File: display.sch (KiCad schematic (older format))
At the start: 122 parts, among them P1 CONN_02X14, P2 CONN_02X15, Q1 BC846, Q10 BC846, Q11 BC856, Q12 BC856, Q13 BC846, Q14 BC846, Q15 BC856, Q16 BC856, Q17 BC846, Q18 BC846, Q19 BC856, Q2 BC846, Q20 BC856, Q21 BC846, Q22 BC846, Q23 BC856, Q24 BC856, Q25 BC846, Q26 BC846, Q27 BC856, Q28 BC856, Q29 BC846, Q3 BC856, Q30 BC846, Q31 BC856, Q32 BC856, Q33 BC846, Q34 BC846, Q35 BC856, Q36 BC856, Q37 BC846, Q38 BC846, Q39 BC856, Q4 BC856, Q40 BC856, Q41 BC846, Q42 BC846, Q43 BC856, Q44 BC856, Q45 BC846, Q46 BC846, Q47 BC856, Q48 BC856, Q5 BC846, Q6 BC846, Q7 BC856, Q8 BC856, Q9 BC846

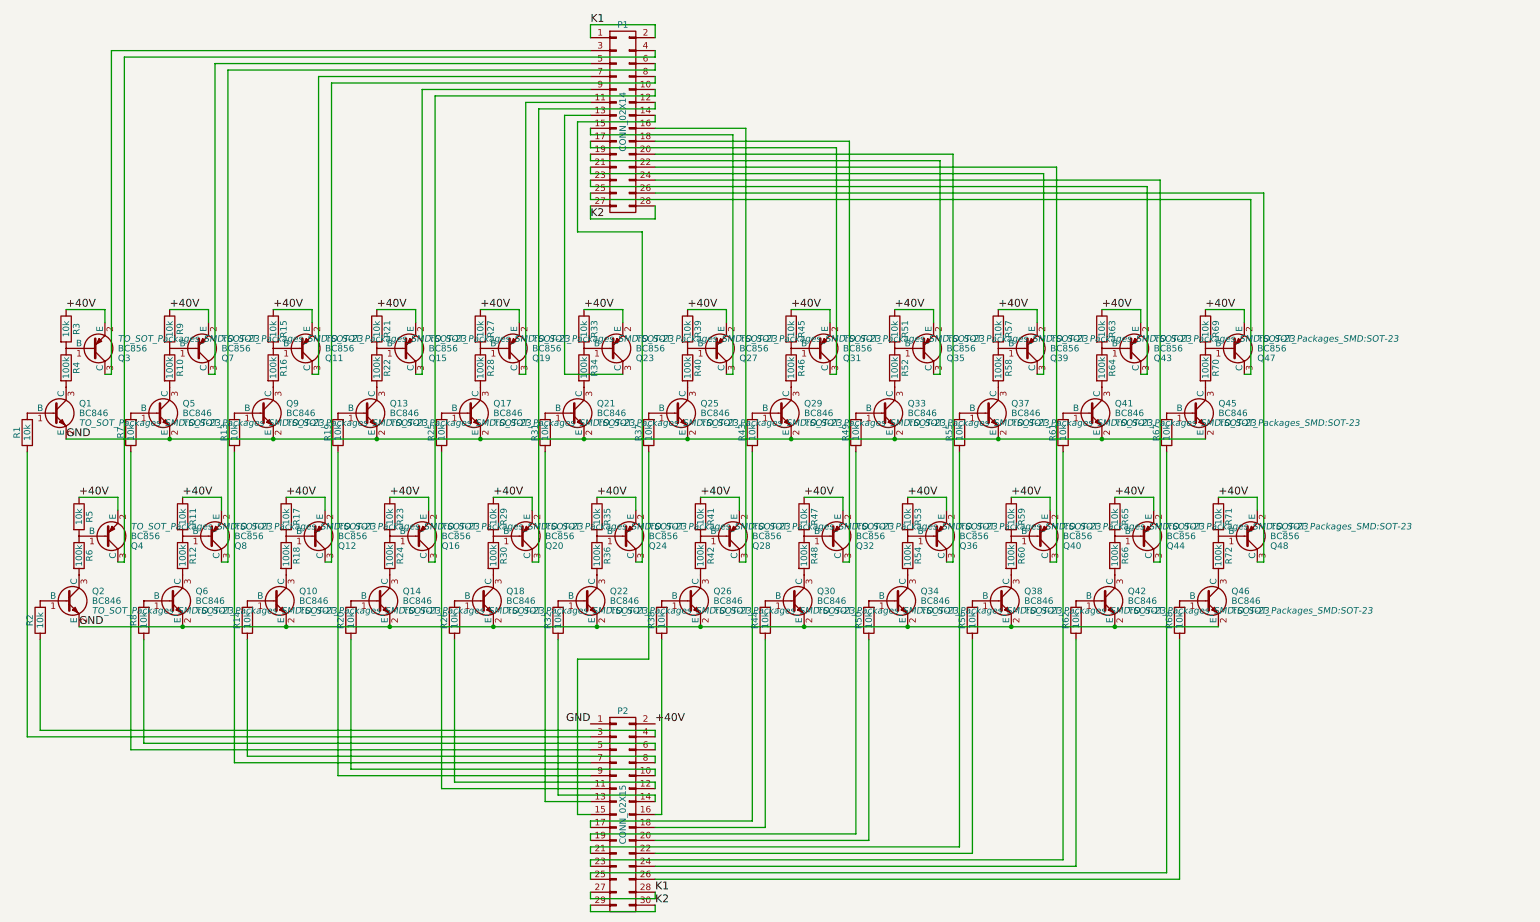
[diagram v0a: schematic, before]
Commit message: Finishing layout, generating gerbers.
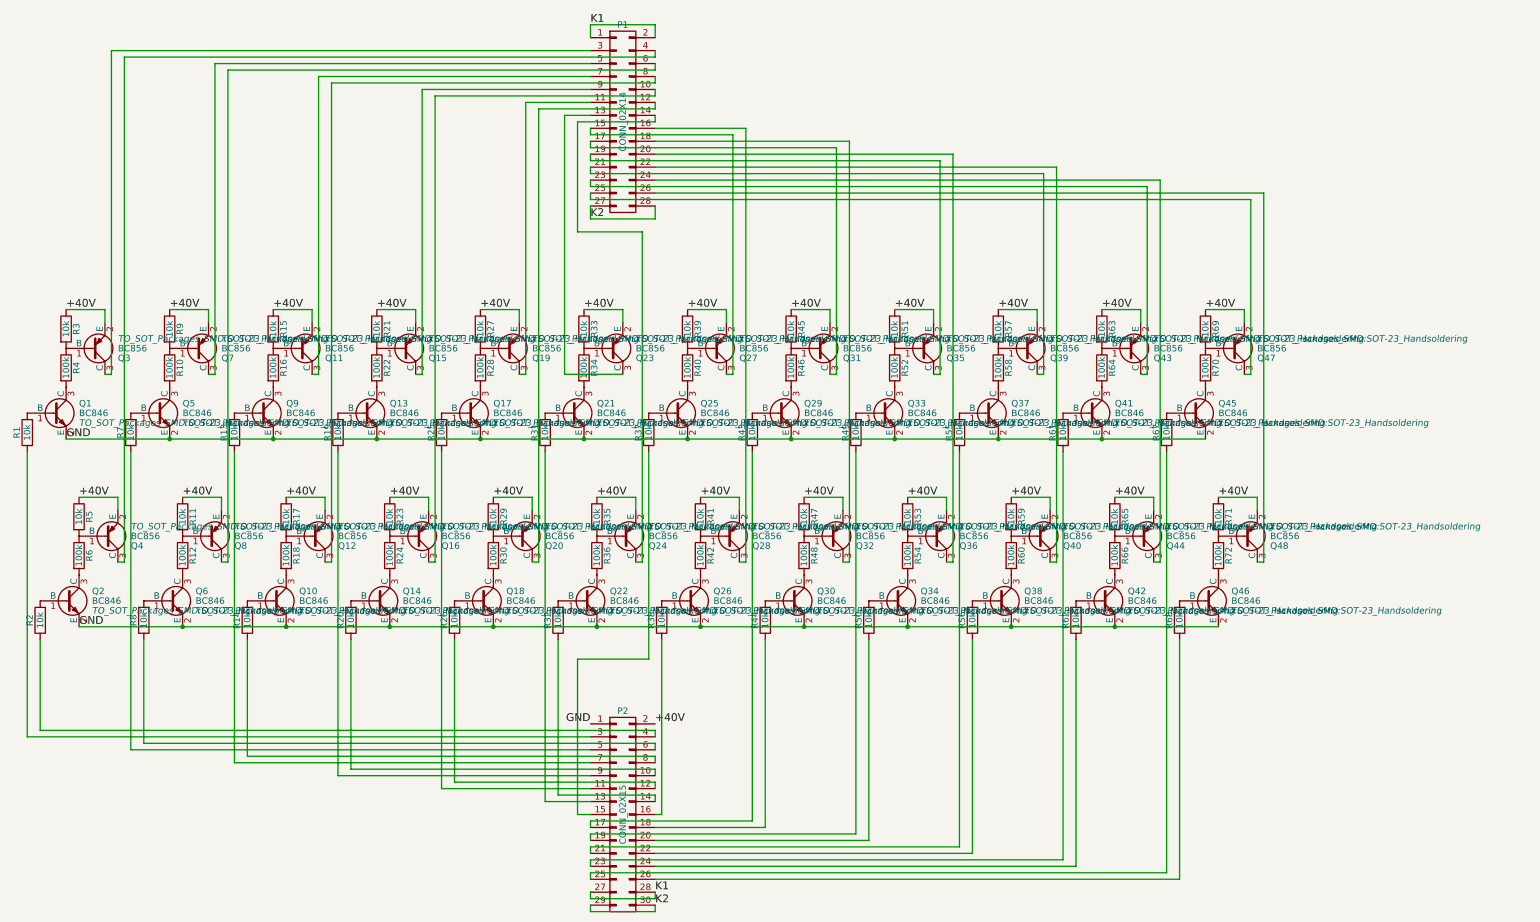
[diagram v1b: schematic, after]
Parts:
- Q1, Q10, Q11, Q12, Q13, Q14, Q15, Q16, Q17, Q18, Q19, Q2, Q20, Q21, Q22, Q23, Q24, Q25, Q26, Q27, Q28, Q29, Q3, Q30, Q31, Q32, Q33, Q34, Q35, Q36, Q37, Q38, Q39, Q4, Q40, Q41, Q42, Q43, Q44, Q45, Q46, Q47, Q48, Q5, Q6, Q7, Q8, Q9: footprint TO_SOT_Packages_SMD:SOT-23 -> TO_SOT_Packages_SMD:SOT-23_Handsoldering
